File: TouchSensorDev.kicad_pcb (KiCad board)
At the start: 2 copper layers, 10 parts, among them J1 Touch, J2 PINS, U1 TTP223-BA6

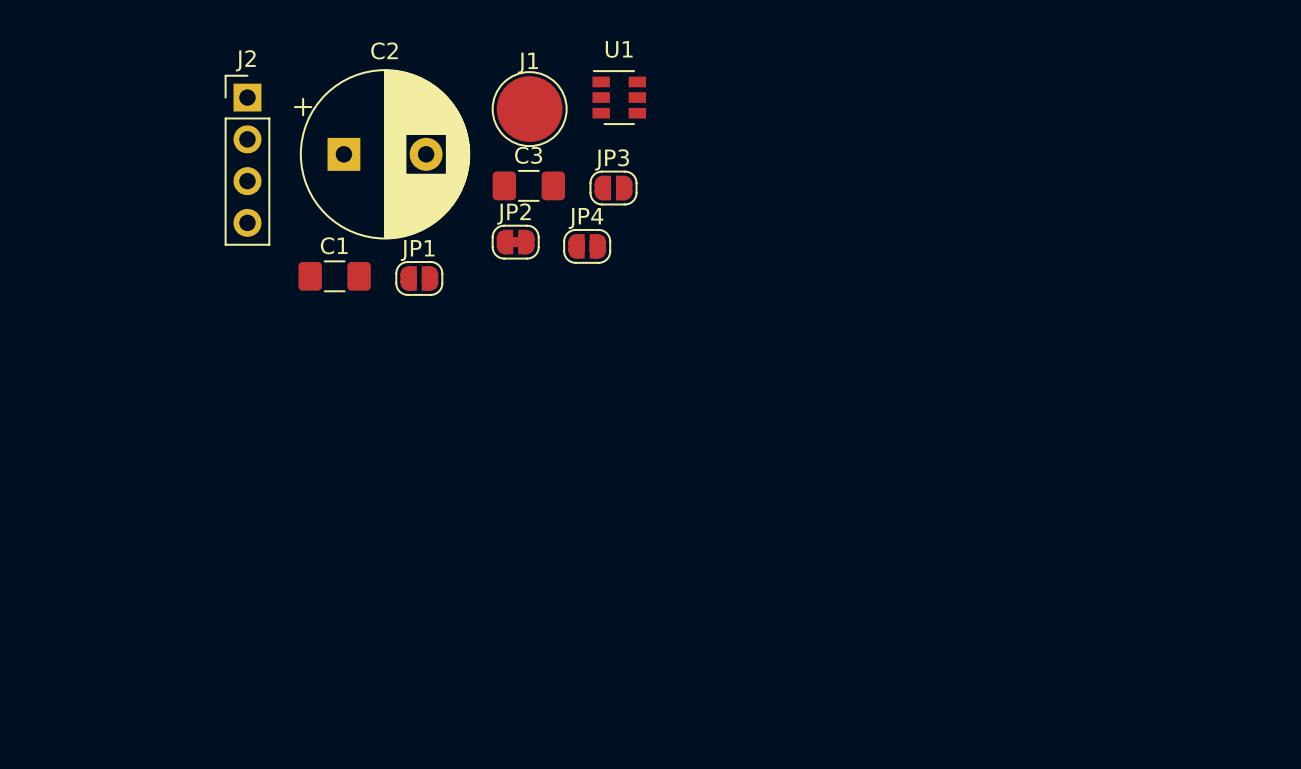
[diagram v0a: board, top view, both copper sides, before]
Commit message: finished board
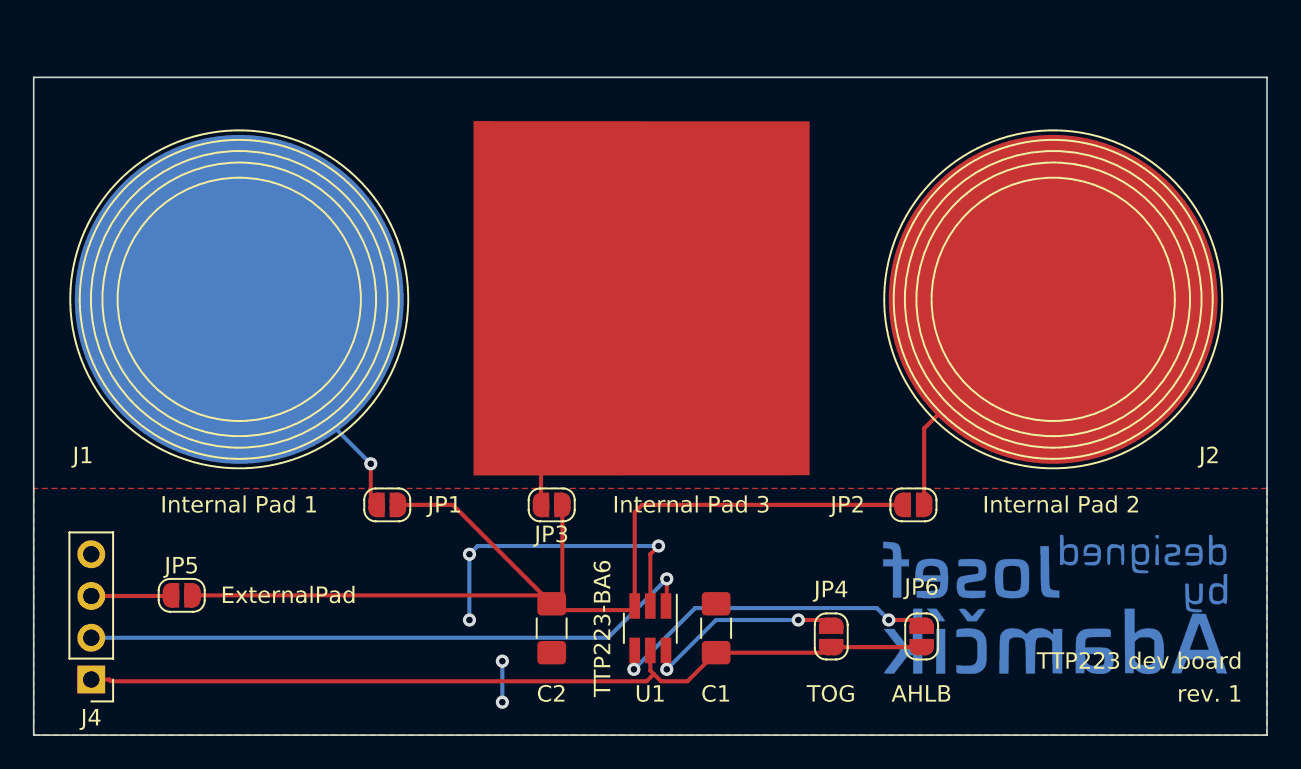
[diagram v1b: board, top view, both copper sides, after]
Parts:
- removed the C2 at (38.9, 24.7)
- removed C3: 0.1u, Capacitor_SMD:C_1206_3216Metric_Pad1.42x1.75mm_HandSolder
- added C1: 0.1u, Capacitor_SMD:C_1206_3216Metric_Pad1.42x1.75mm_HandSolder, F.Cu at (61.5, 53.5)
- added J2: Touch, TouchSensorDev:TouchPadB, F.Cu at (82.0, 33.5)
- added J3: Touch, TouchSensorDev:TouchPadFinger, F.Cu at (57.0, 33.5)
- added JP1: Internal Pad 1, Jumper:SolderJumper-2_P1.3mm_Open_RoundedPad1.0x1.5mm, F.Cu at (41.5, 46.0)
- added JP4: TOG, Jumper:SolderJumper-2_P1.3mm_Open_RoundedPad1.0x1.5mm, F.Cu at (68.5, 54.0)
- added REF**: KiCad-Logo2_5mm_SilkScreen, Symbol:KiCad-Logo2_5mm_SilkScreen, B.Cu at (38.5, 54.5)
- added Ref**: Val**, logos:josef_adamcik_20mm_cu_mask, B.Cu at (82.5, 56.0)
- J1: footprint TestPoint:TestPoint_Pad_D4.0mm -> TouchSensorDev:TouchPadA
- JP2: value InternalPad -> Internal Pad 2; footprint Jumper:SolderJumper-2_P1.3mm_Bridged_RoundedPad1.0x1.5mm -> Jumper:SolderJumper-2_P1.3mm_Open_RoundedPad1.0x1.5mm
- JP3: value TOG -> Internal Pad 3
- U1: footprint Package_TO_SOT_SMD:SOT-23-6 -> Package_TO_SOT_SMD:SOT-23-6_Handsoldering
- moved J4 36.6 mm to (23.5, 56.6), turned to 180 degrees
- moved U1 32.3 mm to (57.5, 53.5), turned to 270 degrees
- moved JP6 31.2 mm to (74.0, 54.0), turned to 270 degrees
- moved JP2 29.0 mm to (73.5, 46.0)
- moved C2 25.1 mm to (51.5, 53.5), turned to 270 degrees
- moved JP5 24.1 mm to (29.0, 51.5)
- moved J1 21.1 mm to (32.5, 33.5)
- moved JP3 19.6 mm to (51.5, 46.0), turned to 180 degrees
- renumbered C1 to C2, J2 to J4, JP1 to JP5, JP4 to JP6
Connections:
- net Net-(J2-Pad2) renamed /OUT
- net Net-(J2-Pad3) renamed /EXTPAD
- net Net-(JP4-Pad1) renamed /AHLB
- C2 pad 1: Net-(C1-Pad1) -> /IN
- JP2 pad 1: Net-(C1-Pad1) -> /IN
- JP2 pad 2: Net-(J1-Pad1) -> Net-(J2-Pad1)
- JP3 pad 1: +5V -> /IN
- JP3 pad 2: Net-(JP3-Pad2) -> Net-(J3-Pad1)
- JP5 pad 2: Net-(C1-Pad1) -> /IN
- U1 pad 3: Net-(C1-Pad1) -> /IN
- U1 pad 6: Net-(JP3-Pad2) -> /TOG
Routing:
- net /IN: track 0.00 -> 68.4 mm
- net +5V: track 0.00 -> 54.4 mm
- net /OUT: track 0.00 -> 38.4 mm, vias 0 -> 1
- net GND: track 0.00 -> 22.1 mm, vias 0 -> 5
- net /AHLB: track 0.00 -> 20.9 mm, vias 0 -> 2
- net Net-(J2-Pad1): track 0.00 -> 16.8 mm
- net Net-(J1-Pad1): track 0.00 -> 16.0 mm, vias 0 -> 1
- net Net-(J3-Pad1): track 0.00 -> 15.0 mm
- net /TOG: track 0.00 -> 12.8 mm, vias 0 -> 2
- net /EXTPAD: track 0.00 -> 4.87 mm
- added copper zone on F.Cu, net GND
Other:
- board outline added: 75 x 40 mm
- board text added: "@josefadamcik"
- board text added: "TTP223 dev board"
- board text added: "https://josef-adamcik.cz"
- board text added: "rev. 1"
